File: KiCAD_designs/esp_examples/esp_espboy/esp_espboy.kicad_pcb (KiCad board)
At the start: 2 copper layers, 74.5 x 72 mm, 32 parts, among them J1 B4B-ZR-SM4-TFT_LF__SN_, J2 B2B-PH-SM4-TBLFSN, J3 Conn_01x02_Pin, J4 B4B-ZR-SM4-TFT_LF__SN_, J5 Conn_01x02_Pin, J6 B7B-ZR-SM4-TFT_LF__SN_, SW1 D2FS-FL-N-A, SW2 RS-282G05A3-SM RT, SW3 RS-282G05A3-SM RT, SW4 D2FS-FL-N-A, U1 ESP-12F, U2 AMS1117-3.3, U3 MCP23017-E_SO

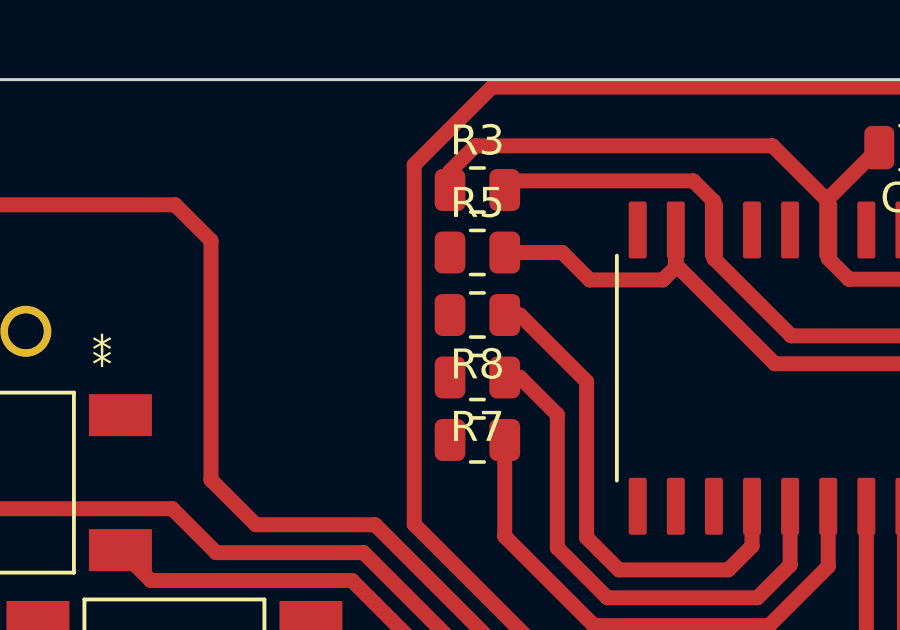
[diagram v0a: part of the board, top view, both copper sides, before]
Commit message: 23017 Updated
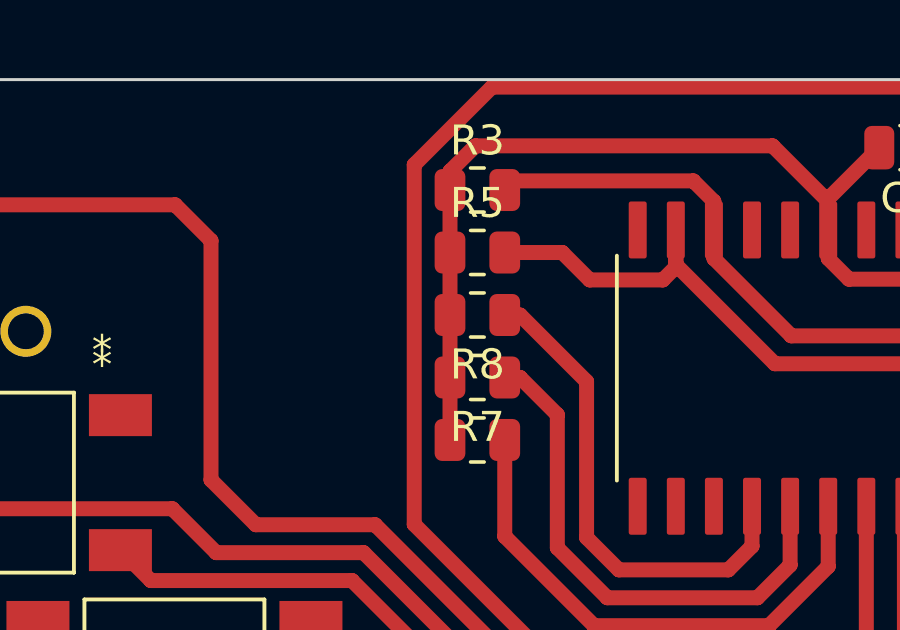
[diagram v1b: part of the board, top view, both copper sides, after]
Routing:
- net VCC: track 237.1 -> 245.5 mm
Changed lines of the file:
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@@
   (segment (start 48.9 48.646) (end 55.849 48.646) (width 0.762) (layer "F.Cu") (net 2))
   (segment (start 53.594 56.642) (end 56.1612 54.0748) (width 0.762) (layer "F.Cu") (net 2))
+  (segment (start 68.4949 67.6808) (end 68.4949 69.7636) (width 0.5) (layer "F.Cu") (net 2))
   (segment (start 78.551 30.796) (end 76.835 32.512) (width 0.762) (layer "F.Cu") (net 2))
   (segment (start 54.517 25.716) (end 49.53 25.716) (width 0.762) (layer "F.Cu") (net 2))
@@
   (segment (start 106.136 76.454) (end 100.167 76.454) (width 0.5) (layer "F.Cu") (net 2))
   (segment (start 84.2778 32.32) (end 84.2778 31.595) (width 0.762) (layer "F.Cu") (net 2))
+  (segment (start 68.4949 73.9292) (end 68.4949 76.012) (width 0.5) (layer "F.Cu") (net 2))
   (segment (start 54.436 41.635) (end 55.025 41.046) (width 0.762) (layer "F.Cu") (net 2))
   (segment (start 81.1022 69.961799) (end 81.1022 69.0118) (width 0.5) (layer "F.Cu") (net 2))
@@
   (segment (start 55.025 26.224) (end 54.517 25.716) (width 0.762) (layer "F.Cu") (net 2))
   (segment (start 49.53 25.716) (end 46.228 29.018) (width 0.762) (layer "F.Cu") (net 2))
+  (segment (start 68.4949 69.7636) (end 68.4949 71.8464) (width 0.5) (layer "F.Cu") (net 2))
   (segment (start 107.12 90.746) (end 108.896 88.97) (width 0.5) (layer "F.Cu") (net 2))
   (segment (start 81.1022 67.9704) (end 81.1022 69.0118) (width 0.5) (layer "F.Cu") (net 2))
@@
   (segment (start 84.2778 32.32) (end 84.2778 35.114) (width 0.762) (layer "F.Cu") (net 2))
   (segment (start 69.342 66.2076) (end 68.4949 67.0547) (width 0.5) (layer "F.Cu") (net 2))
+  (segment (start 68.4949 71.8464) (end 68.4949 73.9292) (width 0.5) (layer "F.Cu") (net 2))
   (segment (start 83.374 30.796) (end 78.551 30.796) (width 0.762) (layer "F.Cu") (net 2))
   (segment (start 76.606399 67.376) (end 70.6247 67.376) (width 0.5) (layer "F.Cu") (net 3))
